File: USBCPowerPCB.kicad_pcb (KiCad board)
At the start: 2 copper layers, 65.2 x 62.2 mm, 109 parts, among them IC2 TPS56A37RPAR, J1 USB_C_Receptacle_PowerOnly_6P, J10 GND_BANANA_OUT, J2 CC, J3 12V_OUT, J4 5V_ISO, J5 5V_OUT, J6 12V_OUT_PIN, J7 5V_ISO_PIN, J8 5V_OUT_PIN, J9 12V_BANANA_OUT, Q1 IRF9358TRPBF, Q2 BSL308PEH6327XTSA1, U1 TVS2200DRV, U2 CYPD3177-24LQXQT, U3 TPS562231DRLR, U4 TPS2116DRL, U5 TBA2-2411

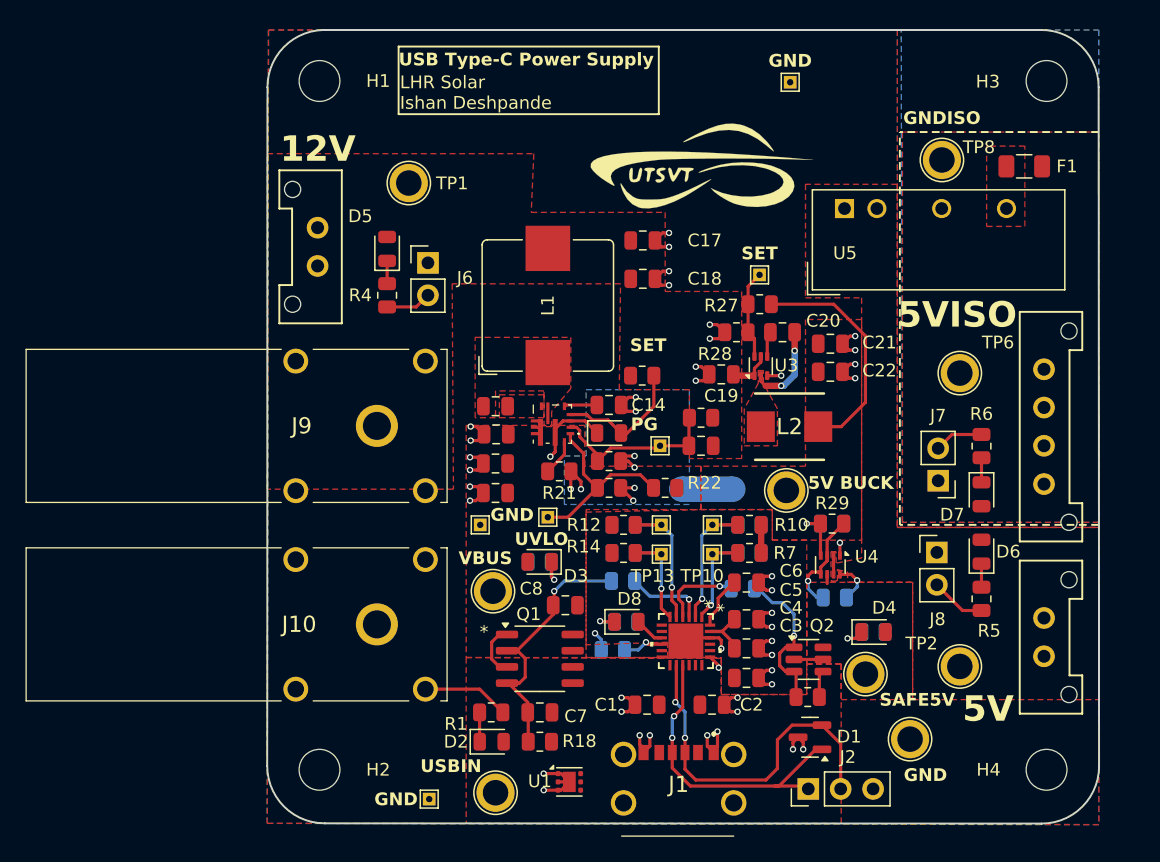
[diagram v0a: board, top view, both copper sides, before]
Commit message: addressed some review comments from my 🐐 champers fu
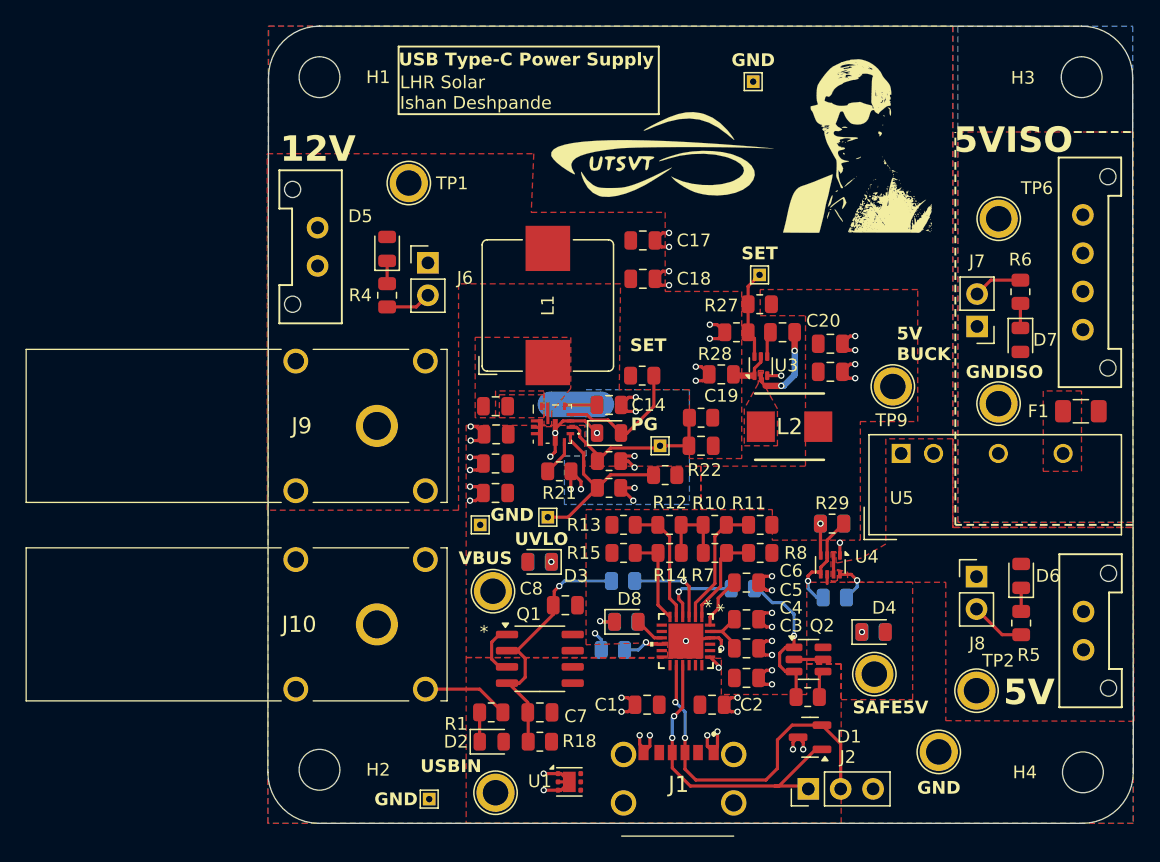
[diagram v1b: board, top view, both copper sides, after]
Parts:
- removed TP10: VBUS_MIN_TP, TestPoint:TestPoint_THTPad_1.0x1.0mm_Drill0.5mm
- removed TP11: VBUS_MAX_TP, TestPoint:TestPoint_THTPad_1.0x1.0mm_Drill0.5mm
- removed TP12: ISNK_COARSE_TP, TestPoint:TestPoint_THTPad_1.0x1.0mm_Drill0.5mm
- removed TP13: ISNK_FINE_TP, TestPoint:TestPoint_THTPad_1.0x1.0mm_Drill0.5mm
- LOGO1: renamed from G***; value LOGO -> UTSVT
- LOGO2: renamed from G***; value LOGO -> Hallock; moved to F.Cu
- LOGO3: renamed from G***; value LOGO -> Troll
- LOGO4: renamed from G***; value LOGO -> Wolf
- R11, R13, R15, R8: moved to F.Cu
- R4: value 5.1k -> 10k
- moved LOGO2 27.6 mm to (155.8, 92.3), turned to 0 degrees
- moved F1 19.7 mm to (173.8, 113.3)
- moved U5 19.7 mm to (159.7, 116.6)
- moved TP8 19.6 mm to (167.3, 112.7)
- moved LOGO4 16.0 mm to (159.2, 104.5)
- moved R6 12.5 mm to (169.1, 103.9)
- moved D7 12.5 mm to (169.1, 107.7)
- moved J7 12.5 mm to (165.7, 106.6)
- moved J4 12.5 mm to (173.9, 97.9)
- moved TP6 12.5 mm to (167.3, 98.2)
- moved LOGO3 12.5 mm to (153.4, 90.2)
- moved NT1 12.3 mm to (134.2, 112.8), turned to 180 degrees
- moved TP9 11.7 mm to (159.1, 111.3), turned to 180 degrees
- moved D6 3.64 mm to (169.1, 126.2)
- moved J8 3.64 mm to (165.6, 126.3)
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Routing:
- net /5V_BUCK: track 26.5 -> 8.40 mm
- net +3.3V: track 8.32 -> 12.3 mm
- net Net-(D3-K): track 2.98 -> 0.03 mm
- net Net-(D4-K): track 2.64 -> 0.03 mm
- net /Power Delivery Controller/ISNK_COARSE: track 11.8 -> 9.59 mm, vias 1 -> 0
- net /5V ORring and Isolator/MUX_SEL: track 4.62 -> 2.48 mm
- net /Power Delivery Controller/ISNK_FINE: track 9.09 -> 7.19 mm, vias 1 -> 0
- net /Power Delivery Controller/VBUS_MAX: track 11.8 -> 9.96 mm, vias 1 -> 0
- net /Power Delivery Controller/VBUS_MIN: track 8.84 -> 7.54 mm, vias 1 -> 0
- net GND: track 79.3 -> 79.9 mm, vias 43 -> 46
- net /Power Delivery Controller/VBUS_FET_EN: track 6.23 -> 6.83 mm
- removed copper zone on F.Cu, net +3.3V
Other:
- board size 65.2 x 62.2 mm -> 67.9 x 62.5 mm
